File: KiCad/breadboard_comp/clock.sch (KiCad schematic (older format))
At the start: 23 parts, among them SW1 SW_Push, SW2 SW_SPDT, U1 LM555, U2 74LS04, U3 74LS08, U4 74LS32, U5 LM555, U6 LM555

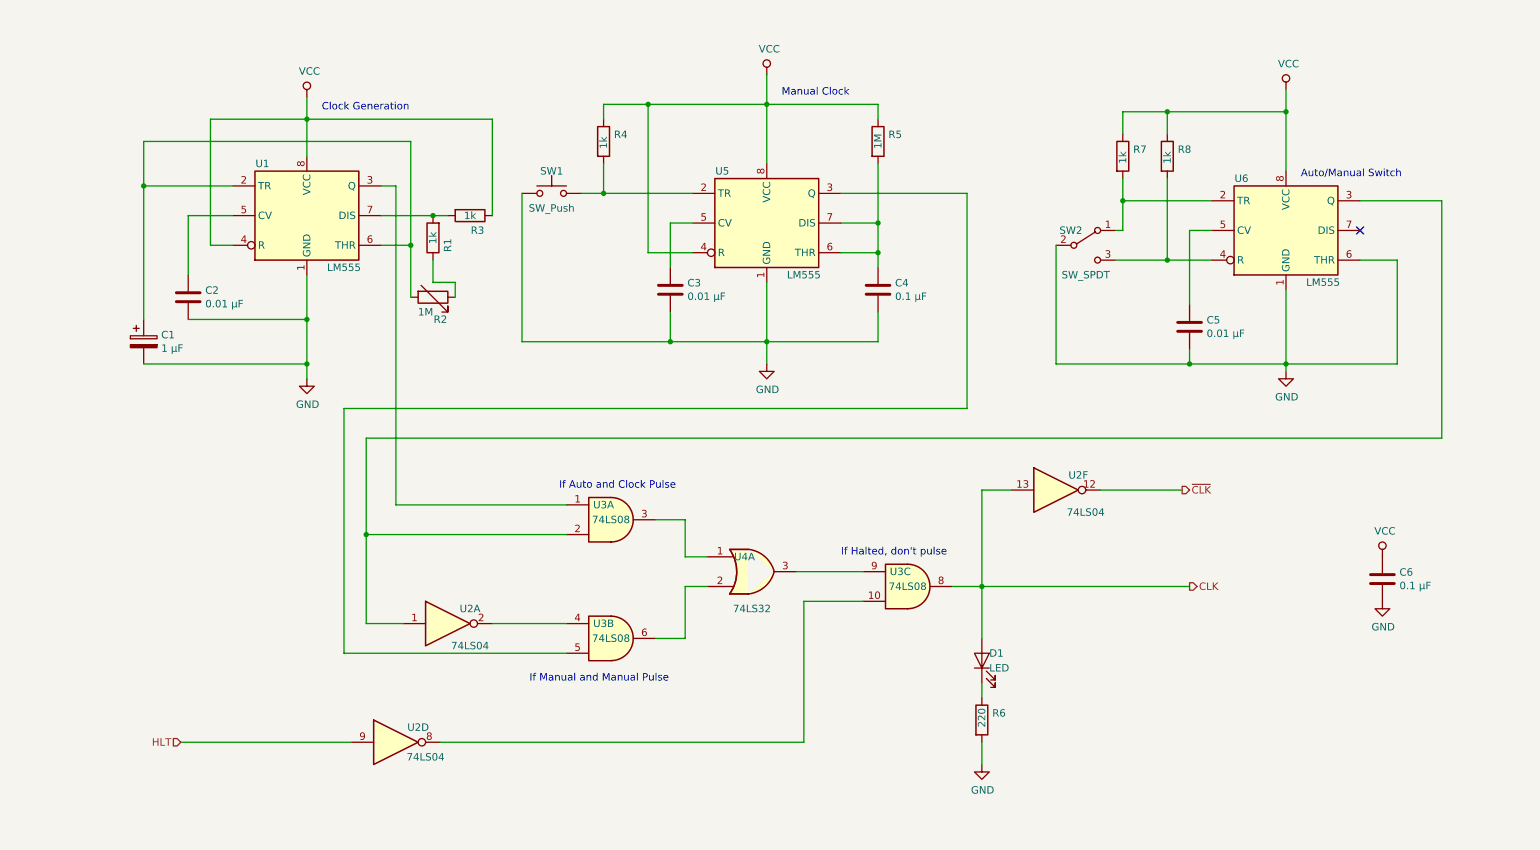
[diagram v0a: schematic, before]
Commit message: Schematic + Report Progress
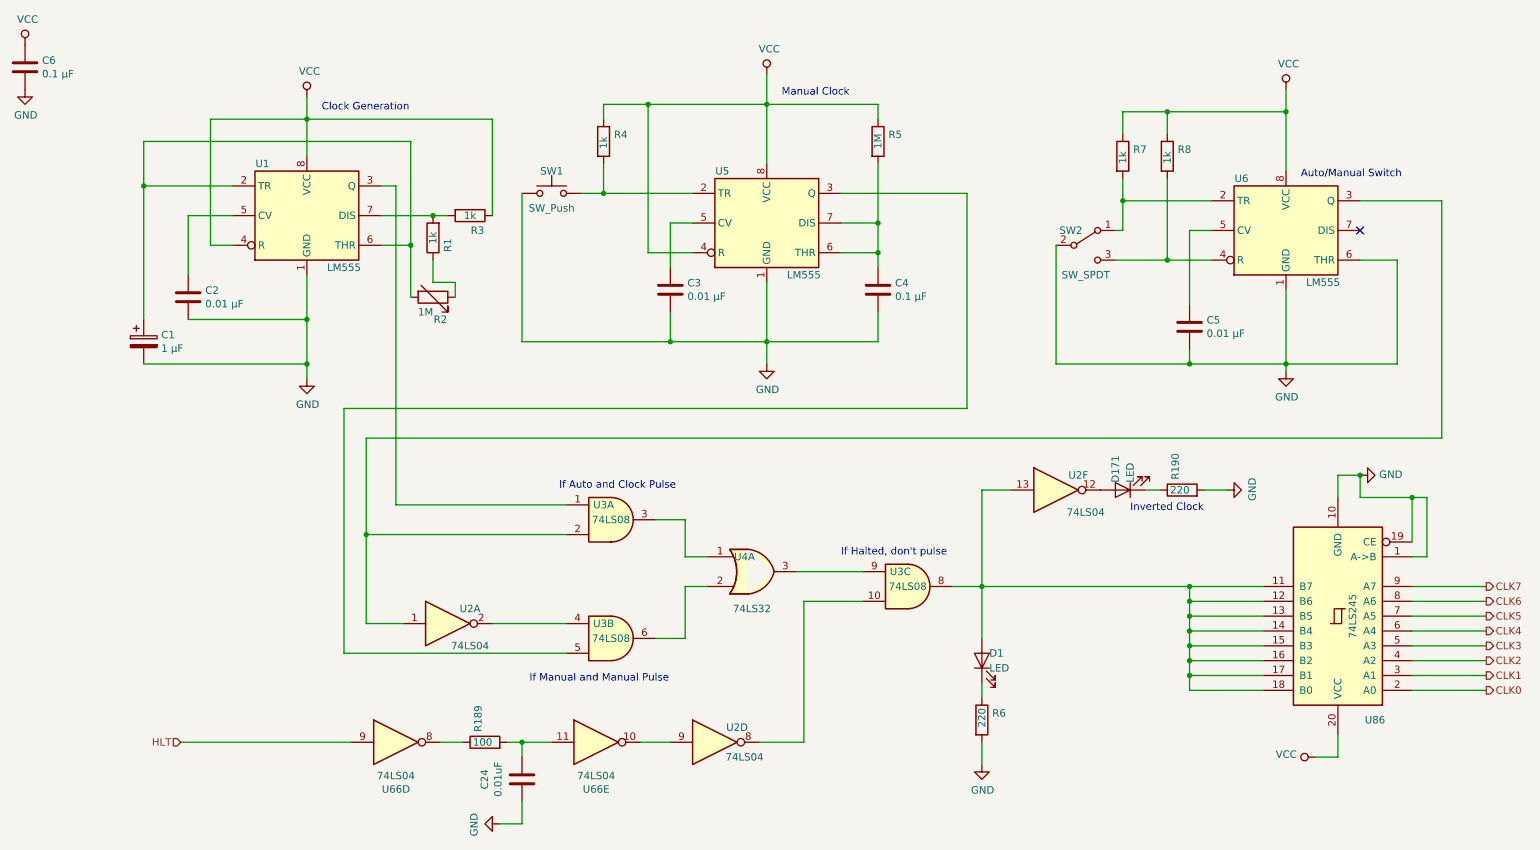
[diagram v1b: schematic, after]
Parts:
- added C24: 0.01uF, symbol Device:C
- added D171: LED, symbol Device:LED
- added R189: 100, symbol Device:R
- added R190: 220, symbol Device:R
- added U66: 74LS04, symbol 74xx:74LS04
- added U86: 74LS245, symbol 74xx:74LS245
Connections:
- net GND: now also C24.2, R190.2, U86.1 (A->B), U86.10 (GND), U86.19 (CE)
- net HLT: now also U66.9; no longer U2.9
- net VCC: now also U86.20 (VCC)
- net CLK: no longer names the net of D1.2 (A), U2.13, U3.8
- net CLK: now also U86.11 (B7), U86.12 (B6), U86.13 (B5), U86.14 (B4), U86.15 (B3), U86.16 (B2), U86.17 (B1), U86.18 (B0)
- net ~CLK: no longer names the net of U2.12
- net ~CLK: now also D171.2 (A)
- new net: U2.9, U66.10
- new net: R189.1, U66.8
- new net: C24.1, R189.2, U66.11
- new net: D171.1 (K), R190.1
- new net CLK0: U86.2 (A0)
- new net CLK1: U86.3 (A1)
- new net CLK2: U86.4 (A2)
- new net CLK3: U86.5 (A3)
- new net CLK4: U86.6 (A4)
- new net CLK5: U86.7 (A5)
- new net CLK6: U86.8 (A6)
- new net CLK7: U86.9 (A7)
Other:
- note added: "Inverted Clock"
- moved on the sheet: C6, U2D
